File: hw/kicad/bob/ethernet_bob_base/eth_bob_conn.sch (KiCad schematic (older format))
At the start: 2 parts, among them P1 CONN_02X25, P2 CONN_02X25

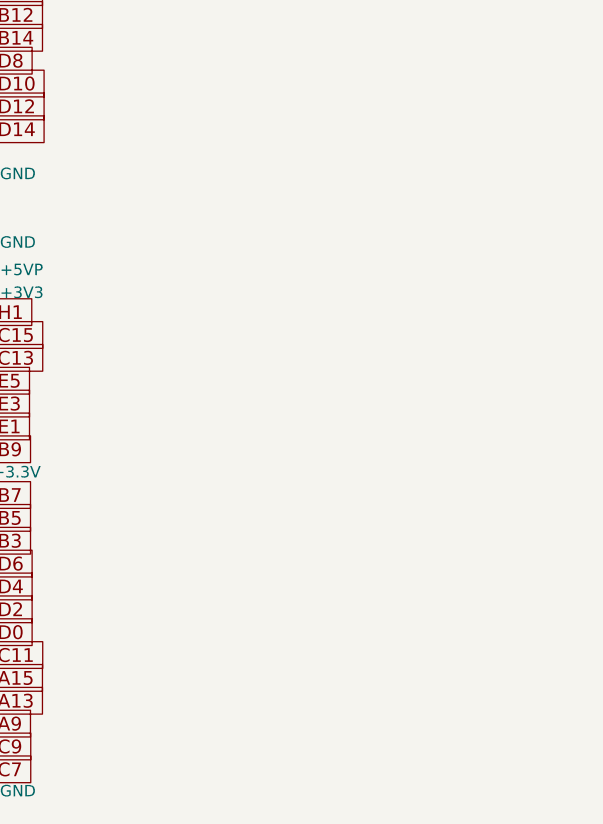
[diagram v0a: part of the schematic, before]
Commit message: add outputs
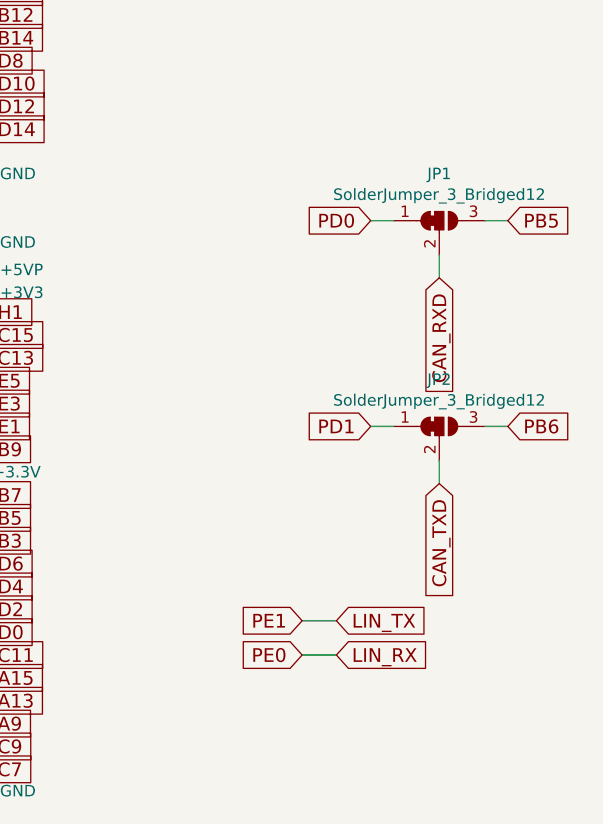
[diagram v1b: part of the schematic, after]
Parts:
- added JP1, JP2: SolderJumper_3_Bridged12, stmbl-kicad-lib:SOLDER_JUMPER_3_NC, symbol Jumper:SolderJumper_3_Bridged12
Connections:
- net PB5: now also JP1.3 (B)
- net PB6: now also JP2.3 (B)
- net PD0: now also JP1.1 (A)
- net PD1: now also JP2.1 (A)
- net PE0 renamed LIN_RX
- net PE1 renamed LIN_TX
- new net CAN_RXD: JP1.2 (C)
- new net CAN_TXD: JP2.2 (C)
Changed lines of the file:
@@
 	0    1    1    0
 $EndComp
+Text GLabel 6600 4100 0    60   Input ~ 0
+PD0
+Text GLabel 6900 4350 3    60   Input ~ 0
+CAN_RXD
+$Comp
+L Jumper:SolderJumper_3_Bridged12 JP1
+U 1 1 5C933169
+P 6900 4100
+F 0 "JP1" H 6900 4305 50  0000 C CNN
+F 1 "SolderJumper_3_Bridged12" H 6900 4214 50  0000 C CNN
+F 2 "stmbl-kicad-lib:SOLDER_JUMPER_3_NC" H 6900 4100 50  0001 C CNN
+F 3 "~" H 6900 4100 50  0001 C CNN
+	1    6900 4100
+	1    0    0    -1
+$EndComp
+Text GLabel 7200 4100 2    60   Input ~ 0
+PB5
+Wire Wire Line
+	6900 4250 6900 4350
+Wire Wire Line
+	6600 4100 6700 4100
+Wire Wire Line
+	7100 4100 7200 4100
+$Comp
+L Jumper:SolderJumper_3_Bridged12 JP2
+U 1 1 5C949A52
+P 6900 5000
+F 0 "JP2" H 6900 5205 50  0000 C CNN
+F 1 "SolderJumper_3_Bridged12" H 6900 5114 50  0000 C CNN
+F 2 "stmbl-kicad-lib:SOLDER_JUMPER_3_NC" H 6900 5000 50  0001 C CNN
+F 3 "~" H 6900 5000 50  0001 C CNN
+	1    6900 5000
+	1    0    0    -1
+$EndComp
+Text GLabel 6600 5000 0    60   Input ~ 0
+PD1
+Wire Wire Line
+	6600 5000 6700 5000
+Text GLabel 7200 5000 2    60   Input ~ 0
+PB6
+Wire Wire Line
+	7200 5000 7100 5000
+Text GLabel 6900 5250 3    60   Input ~ 0
+CAN_TXD
+Wire Wire Line
+	6900 5250 6900 5150
+Text GLabel 6300 5850 0    60   Input ~ 0
+PE1
+Text GLabel 6450 5850 2    60   Input ~ 0
+LIN_TX
+Wire Wire Line
+	6300 5850 6450 5850
+Text GLabel 6300 6000 0    60   Input ~ 0
+PE0
+Text GLabel 6450 6000 2    60   Input ~ 0
+LIN_RX
+Wire Wire Line
+	6300 6000 6450 6000
 $EndSCHEMATC
